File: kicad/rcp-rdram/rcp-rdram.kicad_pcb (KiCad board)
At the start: 2 copper layers, 64.8 x 51.2 mm, 29 parts, among them P1 RDRAM-EDGE, U11 RDRAM18-NUS, U11-2 RDRAM18-NUS, U14 RDRAM18-NUS, U14-2 RDRAM18-NUS, U15 MX8330, X2 14.705MHz

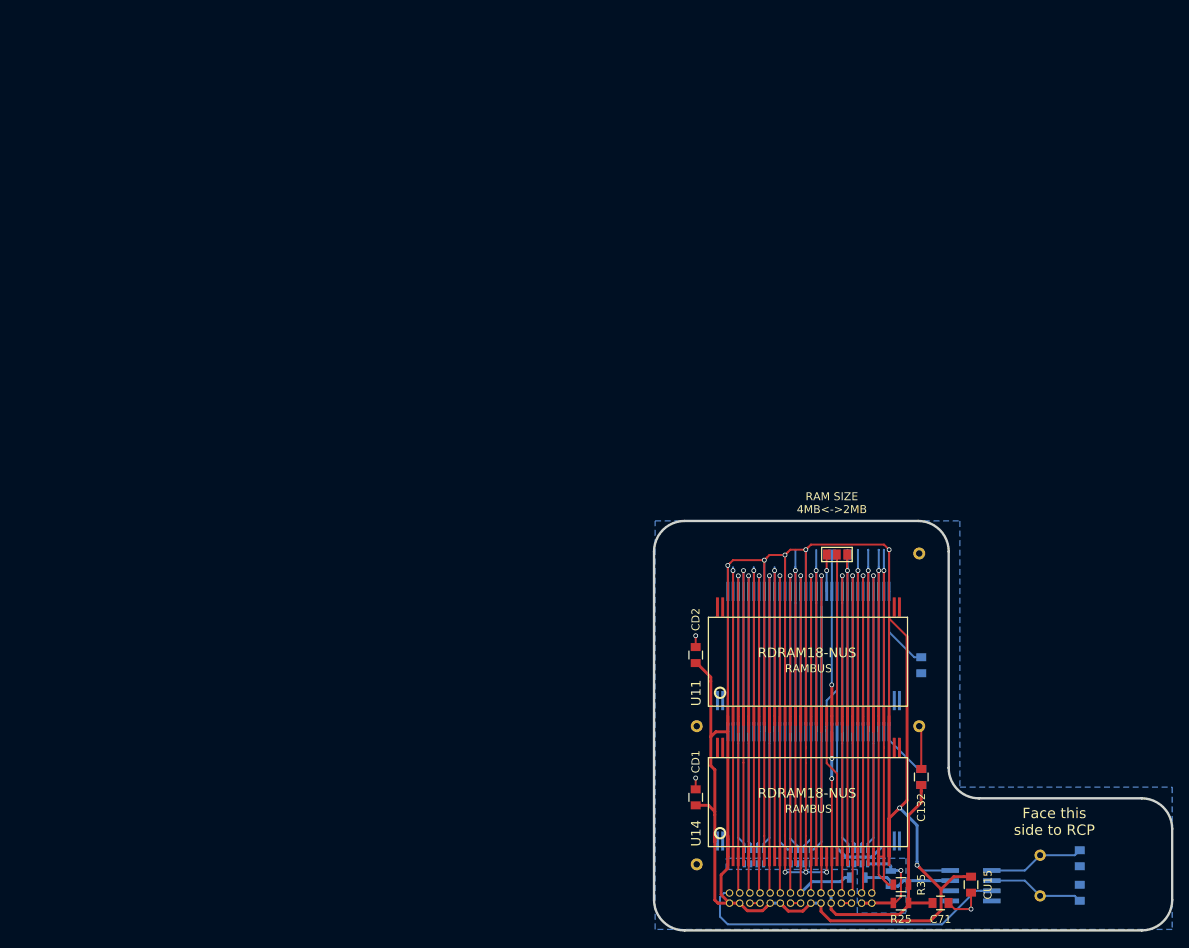
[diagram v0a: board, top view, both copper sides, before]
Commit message: Revision 2, mostly finished, TODO: checks
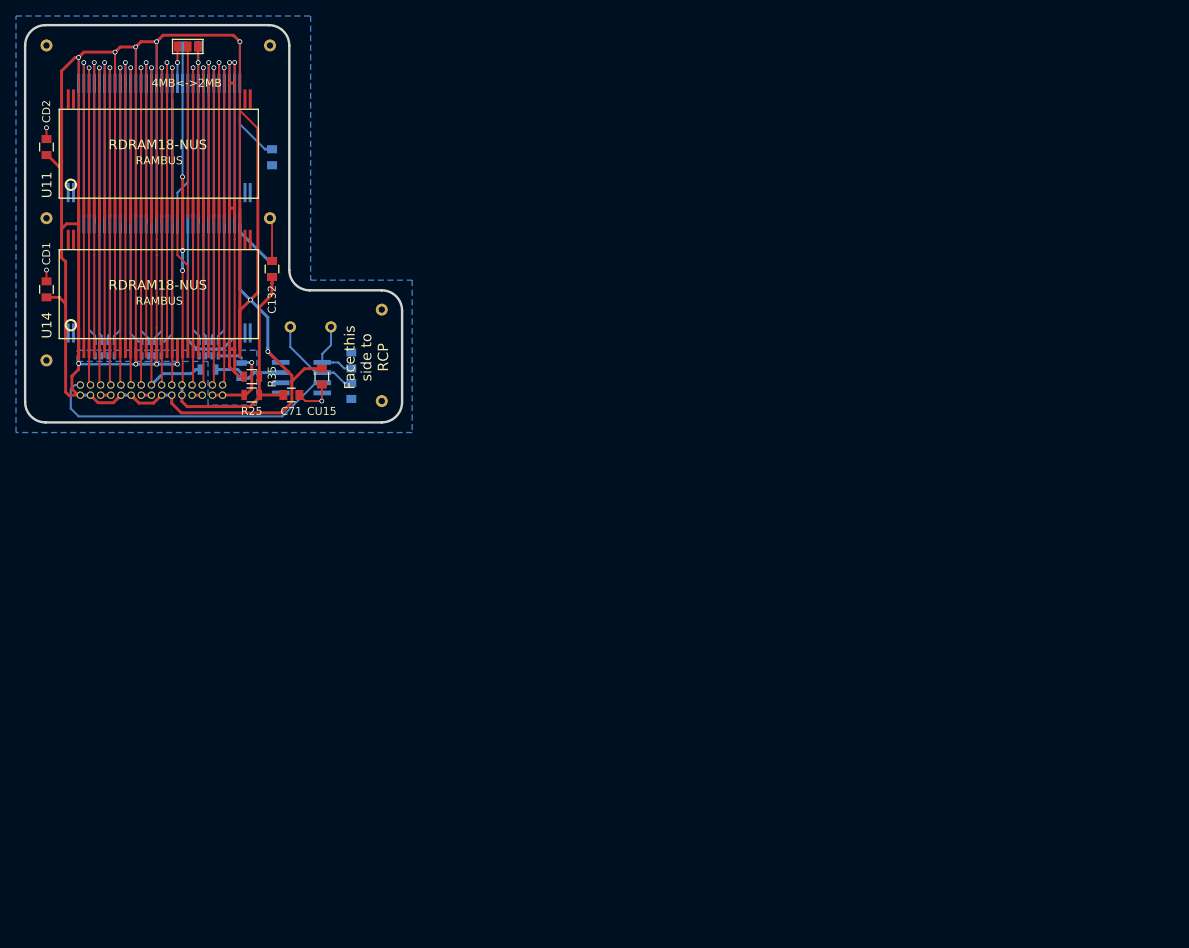
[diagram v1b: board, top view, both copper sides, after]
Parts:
- added REF**: MountingHole_2.2mm_M2_DIN965_Pad, Mounting_Holes:MountingHole_2.2mm_M2_DIN965_Pad, F.Cu at (67.4, 64.8)
- added REF**: MountingHole_2.2mm_M2_DIN965_Pad, Mounting_Holes:MountingHole_2.2mm_M2_DIN965_Pad, F.Cu at (67.4, 53.3)
- added REF**: MountingHole_2.2mm_M2_DIN965_Pad, Mounting_Holes:MountingHole_2.2mm_M2_DIN965_Pad, F.Cu at (25.5, 20.3)
- moved C146 110.6 mm to (63.6, 63.5), turned to 270 degrees
- moved X2 110.5 mm to (61.1, 55.5), turned to 180 degrees
- moved C147 110.3 mm to (63.6, 59.7), turned to 90 degrees
- moved U15 105.1 mm to (57.4, 61.8)
- moved REF** 103.1 mm to (25.5, 41.9)
- moved C71 103.0 mm to (56.1, 64.0)
- moved CD1 103.0 mm to (25.5, 50.8)
- moved R25 103.0 mm to (51.2, 64.0)
- moved R33 103.0 mm to (45.7, 60.8)
- moved REF** 103.0 mm to (53.5, 41.9)
- moved U11 103.0 mm to (39.6, 34.7)
- moved U11-2 103.0 mm to (39.6, 48.6)
- moved U14 103.0 mm to (39.6, 52.3)
- moved C132 103.0 mm to (53.7, 48.3)
- moved C133 103.0 mm to (43.6, 20.4)
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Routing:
- net VDD: track 484.4 -> 514.8 mm, vias 10 -> 11
- net GND: track 688.0 -> 672.5 mm
- net Net-(C147-Pad1): track 12.0 -> 8.83 mm
- net Net-(R32-Pad1): track 11.8 -> 9.22 mm
- net Net-(P1-Pad15): track 40.2 -> 37.7 mm
- net /VTERM: track 13.5 -> 12.9 mm
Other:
- board size 64.8 x 51.2 mm -> 47.1 x 49.7 mm
- board text added: "4MB<->2MB"
- board text removed: "RAM SIZE 4MB<->2MB"
